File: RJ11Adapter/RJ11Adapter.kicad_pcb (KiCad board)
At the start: 2 copper layers, 31 x 21 mm, 4 parts, among them J1 RAIN_GAUGE, J2 WIND_RAIN, J3 WIND

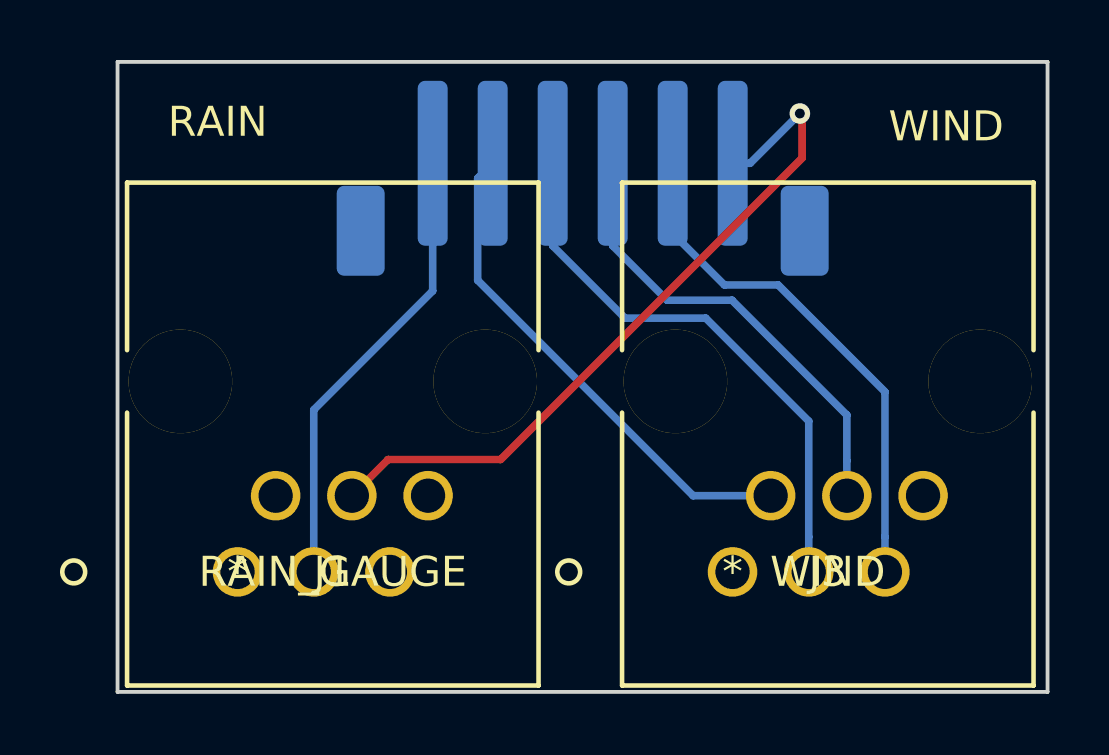
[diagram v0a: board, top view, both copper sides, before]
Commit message: New A-2014-1-4-N-T-R Footprint
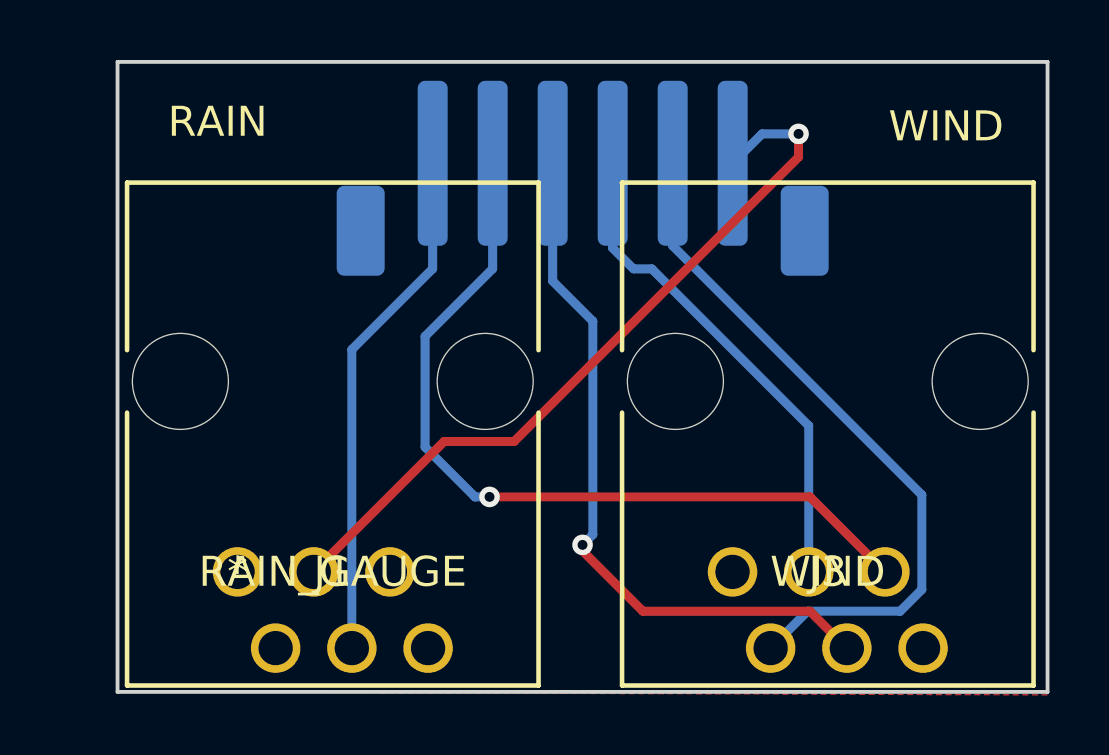
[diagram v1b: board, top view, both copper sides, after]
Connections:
- J1 pad 1: (no net) -> Net-(J1-Pad1)
- J1 pad 2: (no net) -> Net-(J1-Pad2)
- J1 pad 5: (no net) -> Net-(J1-Pad5)
- J1 pad 6: (no net) -> Net-(J1-Pad6)
- J3 pad 1: (no net) -> Net-(J3-Pad1)
- J3 pad 6: (no net) -> Net-(J3-Pad6)
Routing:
- net /VANE_A: track 16.8 -> 27.4 mm, vias 0 -> 1
- net /VANE_B: track 17.6 -> 23.5 mm
- net /ANEM_A: track 18.7 -> 23.8 mm, vias 0 -> 1
- net /RAIN_A: track 15.3 -> 17.3 mm
- net /RAIN_B: track 24.1 -> 25.3 mm
- net /ANEM_B: track 15.6 -> 16.7 mm
- added copper zone on B.Cu, net (none)
- added copper zone on F.Cu, net (none)
